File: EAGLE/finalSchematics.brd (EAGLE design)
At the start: 60 x 60 mm, 35 parts, among them IC1 STM32F103RBT, J2 U.FL, J3 U.FL, U1 LM1117-3.3

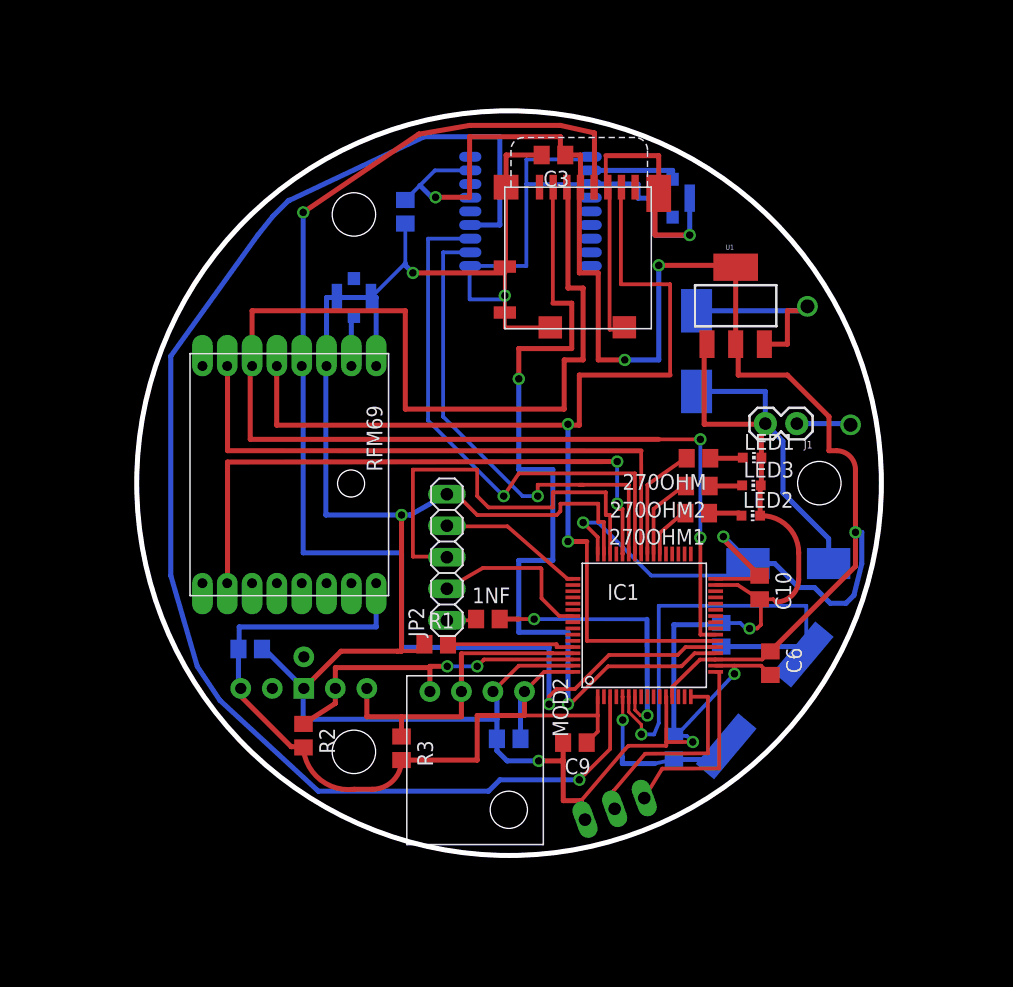
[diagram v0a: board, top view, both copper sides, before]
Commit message: Final fixes before etching
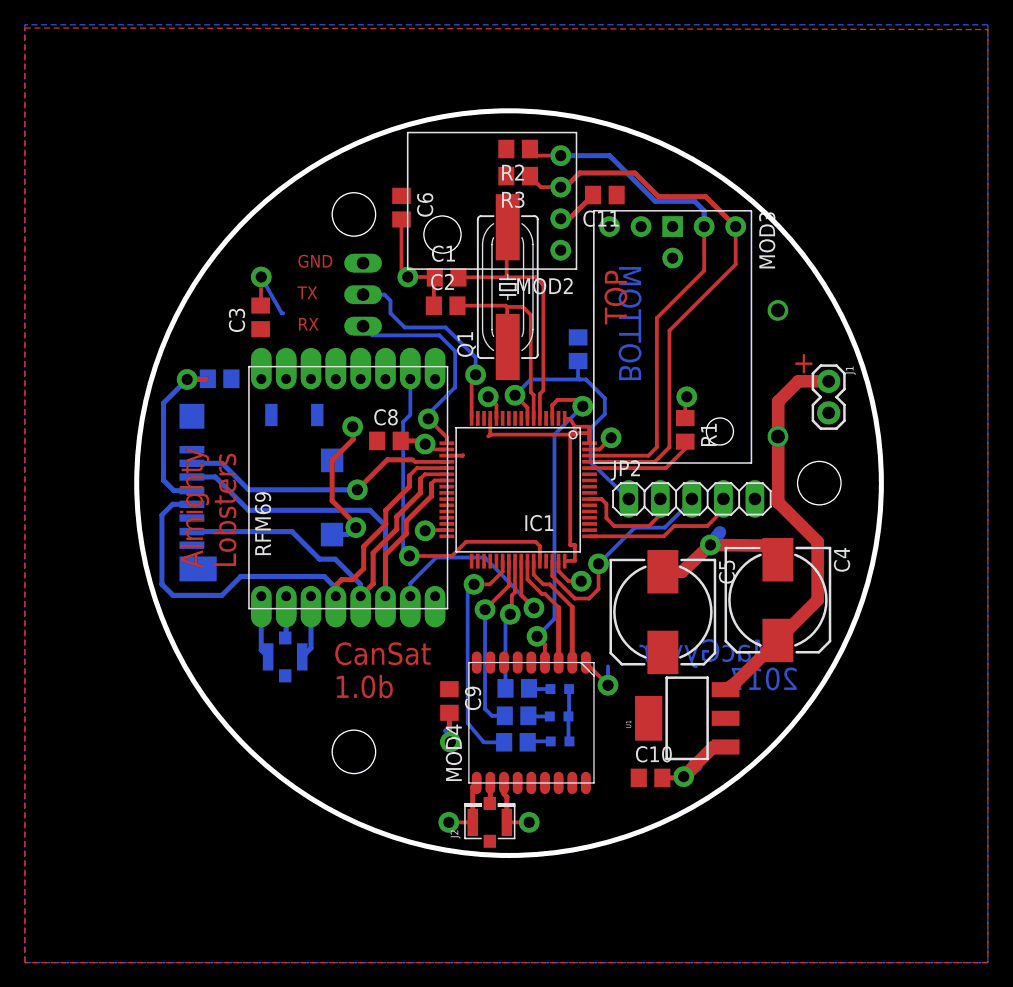
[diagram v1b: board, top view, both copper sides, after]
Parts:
- removed 1NF: (no value), rcl:C0805
- removed 270OHM, 270OHM1, 270OHM2: (no value), resistor:R0805
- added C12: 1n, rcl:C0805
- added R4, R5, R6: 270, resistor:R0805
- C1, C2: value 4.7p 906-099 -> 15p
- C10, C11, C3, C6, C7, C8, C9: value (none) -> 100n
- J1: value (none) -> PWR
- JP1: value (none) -> DBG
- JP2: value (none) -> SWD
- LED1, LED2, LED3: value (none) -> GRN
- Q1: value (none) -> 8 MHz
- SD1: value (none) -> SD
- moved J2 52.4 mm to (28.4, 2.67), flipped to the top
- moved R2 50.3 mm to (30.7, 56.9), turned to 180 degrees
- moved MOD3 47.6 mm to (43.2, 50.7), flipped to the top, turned to 270 degrees
- moved C6 47.2 mm to (21.3, 52.2)
- moved R3 47.0 mm to (30.7, 54.7), turned to 180 degrees
- moved JP1 46.1 mm to (18.2, 45.2), turned to 90 degrees
- moved MOD2 45.1 mm to (35.4, 57.7), turned to 180 degrees
- moved C11 44.5 mm to (37.7, 53.2), flipped to the top, turned to 180 degrees
- moved C1 42.1 mm to (25.0, 46.6), flipped to the top, turned to 0 degrees
- moved MOD4 41.7 mm to (36.2, 5.84), flipped to the top, turned to 90 degrees
- moved SD1 39.5 mm to (4.45, 29.6), flipped to the bottom, turned to 90 degrees
- moved Q1 39.2 mm to (29.9, 45.8), flipped to the top, turned to 90 degrees
- moved C2 34.6 mm to (24.9, 44.3), flipped to the top, turned to 0 degrees
- moved U1 33.5 mm to (44.3, 11.0), turned to 90 degrees
- moved J3 29.5 mm to (12.0, 16.0), turned to 90 degrees
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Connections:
- removed net N$4: D1.A, J1.1
- removed net N$8: 1NF.2, IC1.7
- net GND: now also C12.1, D1.A
- net N$10: now also R4.2; no longer 270OHM.2
- net N$11: now also R4.1; no longer 270OHM.1
- net N$12: now also R6.1; no longer 270OHM1.1
- net N$13: now also R5.1; no longer 270OHM2.1
- net N$3: now also J1.1
- net N$7: now also R6.2; no longer 270OHM1.2
- net N$9: now also R5.2; no longer 270OHM2.2
- net NRST: now also C12.2, IC1.7; no longer 1NF.1
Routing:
- net GND: track 341.0 -> 99.6 mm, vias 8 -> 16
- net +3V3: track 229.4 -> 42.4 mm, vias 6 -> 1
- net 1PPS: track 112.1 -> 26.5 mm, vias 1 -> 2
- net MOSI: track 117.5 -> 34.9 mm, vias 2 -> 0
- net SCK: track 105.2 -> 40.4 mm, vias 2 -> 0
- net MISO: track 89.1 -> 30.0 mm, vias 2 -> 0
- net CS-SD: track 70.5 -> 22.5 mm, vias 2 -> 1
- net RX: track 44.7 -> 9.36 mm, vias 1 -> 0
- net CS-RAD: track 48.5 -> 17.8 mm, vias 0 -> 1
- net TX: track 39.8 -> 9.76 mm, vias 1 -> 0
- net DIO0: track 49.2 -> 27.0 mm, vias 2 -> 1
- net N$8: track 21.9 -> 0.00 mm, vias 2 -> 0
- net SCL: track 25.9 -> 46.1 mm
- net NRST: track 2.45 -> 22.1 mm, vias 0 -> 1
- net N$1: track 40.2 -> 21.5 mm, vias 1 -> 0
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- added copper zone on layer 1, net +3V3
- added copper zone on layer 16, net GND
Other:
- board text added: "+"
- board text added: "2017"
- board text added: "Almighty Lobsters"
- board text added: "BOTTOM"
- board text added: "CanSat 1.0b"
- board text added: "GND TX RX"
- board text added: "MacGyver"
- board text added: "TOP"
- board text added: "bSTOP"
- board text added: "tSTOP"
